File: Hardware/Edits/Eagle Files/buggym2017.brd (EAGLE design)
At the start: 88.9 x 81.3 mm, 6 parts, among them IC1 4001N, IC2 4075N, IC3 BCC, IC4 L293E

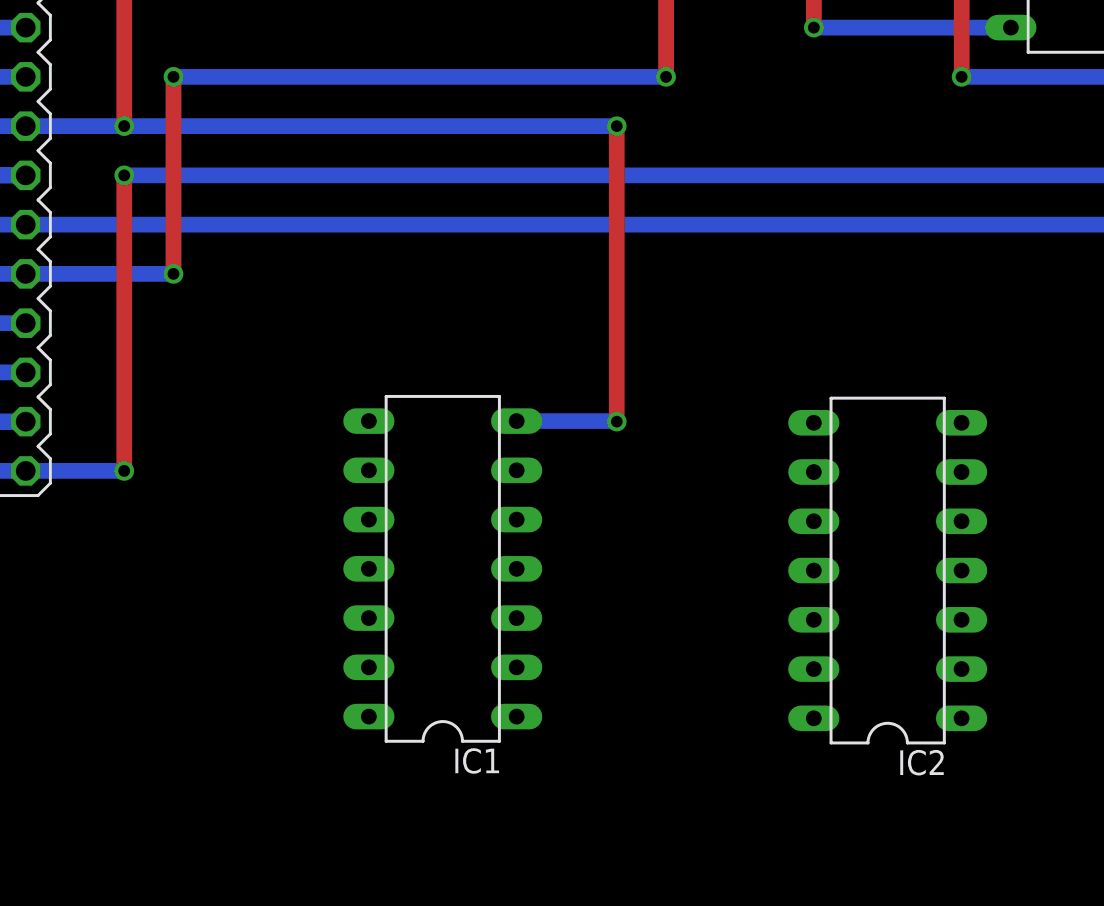
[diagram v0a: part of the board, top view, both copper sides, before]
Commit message: Work Done in Week 3  HardwareLab
Work done in Multisim and Eagle
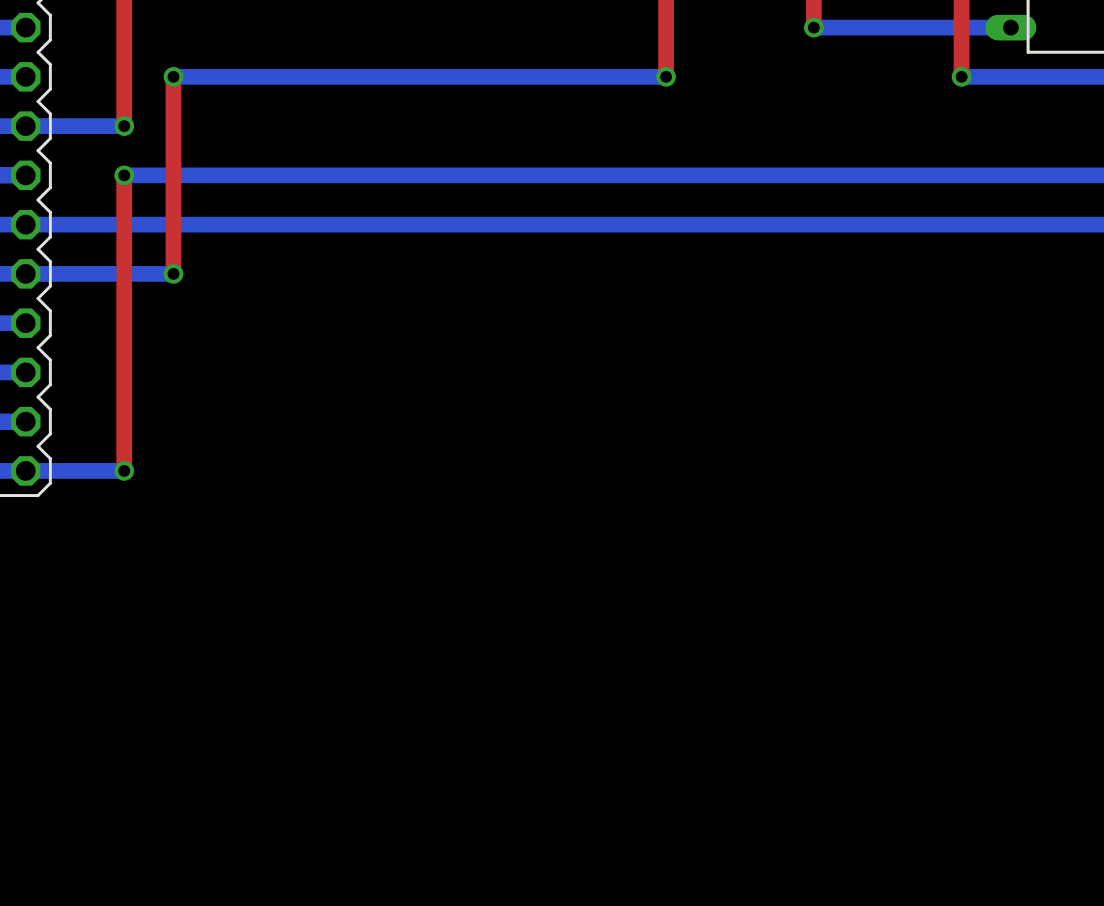
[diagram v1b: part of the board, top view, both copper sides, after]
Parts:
- removed IC1: 4001N, 40xx:DIL14
- removed IC2: 4075N, 40xx:DIL14
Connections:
- removed net LM: IC2.9
- removed net N$1: IC1.3, IC2.2
- removed net N$4: IC1.4, IC2.4
- removed net RM: IC2.6
- removed net VDD: IC1.14, IC2.14
- net GND: no longer IC1.7, IC2.7
- net L_EYE: no longer BUGGY_CON.4
- net R_EYE: no longer BUGGY_CON.3
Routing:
- net GND: track 159.9 -> 94.0 mm, vias 8 -> 6
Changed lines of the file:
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@@
 <?xml version="1.0" encoding="utf-8"?>
 <!DOCTYPE eagle SYSTEM "eagle.dtd">
-<eagle version="7.7.0">
+<eagle version="7.3.0">
 <drawing>
 <settings>
@@
 <setting verticaltext="up"/>
 </settings>
-<grid distance="0.1" unitdist="inch" unit="inch" style="lines" multiple="1" display="yes" altdistance="0.01" altunitdist="inch" altunit="inch"/>
+<grid distance="0.1" unitdist="inch" unit="inch" style="lines" multiple="1" display="yes" altdistance="0.025" altunitdist="inch" altunit="inch"/>
 <layers>
 <layer number="1" name="Top" color="4" fill="1" visible="yes" active="yes"/>
@@
 <layer number="27" name="tValues" color="7" fill="1" visible="yes" active="yes"/>
 <layer number="28" name="bValues" color="7" fill="1" visible="yes" active="yes"/>
-<layer number="29" name="tStop" color="7" fill="3" visible="yes" active="yes"/>
-<layer number="30" name="bStop" color="7" fill="6" visible="yes" active="yes"/>
-<layer number="31" name="tCream" color="7" fill="4" visible="yes" active="yes"/>
-<layer number="32" name="bCream" color="7" fill="5" visible="yes" active="yes"/>
-<layer number="33" name="tFinish" color="6" fill="3" visible="yes" active="yes"/>
-<layer number="34" name="bFinish" color="6" fill="6" visible="yes" active="yes"/>
-<layer number="35" name="tGlue" color="7" fill="4" visible="yes" active="yes"/>
-<layer number="36" name="bGlue" color="7" fill="5" visible="yes" active="yes"/>
-<layer number="37" name="tTest" color="7" fill="1" visible="yes" active="yes"/>
-<layer number="38" name="bTest" color="7" fill="1" visible="yes" active="yes"/>
+<layer number="29" name="tStop" color="7" fill="3" visible="no" active="yes"/>
+<layer number="30" name="bStop" color="7" fill="6" visible="no" active="yes"/>
+<layer number="31" name="tCream" color="7" fill="4" visible="no" active="yes"/>
+<layer number="32" name="bCream" color="7" fill="5" visible="no" active="yes"/>
+<layer number="33" name="tFinish" color="6" fill="3" visible="no" active="yes"/>
+<layer number="34" name="bFinish" color="6" fill="6" visible="no" active="yes"/>
+<layer number="35" name="tGlue" color="7" fill="4" visible="no" active="yes"/>
+<layer number="36" name="bGlue" color="7" fill="5" visible="no" active="yes"/>
+<layer number="37" name="tTest" color="7" fill="1" visible="no" active="yes"/>
+<layer number="38" name="bTest" color="7" fill="1" visible="no" active="yes"/>
 <layer number="39" name="tKeepout" color="4" fill="11" visible="yes" active="yes"/>
 <layer number="40" name="bKeepout" color="1" fill="11" visible="yes" active="yes"/>
@@
 <layer number="42" name="bRestrict" color="1" fill="10" visible="yes" active="yes"/>
 <layer number="43" name="vRestrict" color="2" fill="10" visible="yes" active="yes"/>
-<layer number="44" name="Drills" color="7" fill="1" visible="yes" active="yes"/>
-<layer number="45" name="Holes" color="7" fill="1" visible="yes" active="yes"/>
-<layer number="46" name="Milling" color="3" fill="1" visible="yes" active="yes"/>
-<layer number="47" name="Measures" color="7" fill="1" visible="yes" active="yes"/>
+<layer number="44" name="Drills" color="7" fill="1" visible="no" active="yes"/>
+<layer number="45" name="Holes" color="7" fill="1" visible="no" active="yes"/>
+<layer number="46" name="Milling" color="3" fill="1" visible="no" active="yes"/>
+<layer number="47" name="Measures" color="7" fill="1" visible="no" active="yes"/>
 <layer number="48" name="Document" color="7" fill="1" visible="yes" active="yes"/>
 <layer number="49" name="Reference" color="7" fill="1" visible="yes" active="yes"/>
@@
 </element>
 <element name="BUGGY_CON" library="2E10" package="2E10BOARD" value="2E10HDR" x="26.67" y="38.1"/>
-<element name="IC1" library="40xx" package="DIL14" value="4001N" x="49.44543125" y="17.810665625" rot="R90"/>
-<element name="IC2" library="40xx" package="DIL14" value="4075N" x="72.387890625" y="17.722265625" rot="R90"/>
 </elements>
 <signals>
@@
 <wire x1="27.94" y1="53.34" x2="43.18" y2="53.34" width="0.8128" layer="16"/>
 <via x="45.72" y="53.34" extent="1-16" drill="0.6096" shape="square"/>
-<contactref element="IC1" pad="7"/>
-<contactref element="IC2" pad="7"/>
-<wire x1="33.02" y1="40.64" x2="52.944703125" y2="40.64" width="0.4064" layer="16"/>
-<wire x1="52.944703125" y1="40.64" x2="52.944703125" y2="40.489321875" width="0.4064" layer="16"/>
-<wire x1="53.25543125" y1="25.430665625" x2="58.42" y2="25.430665625" width="0.8128" layer="16"/>
-<wire x1="58.42" y1="25.430665625" x2="58.42" y2="25.4" width="0.8128" layer="16"/>
-<via x="58.42" y="25.4" extent="1-16" drill="0.6" shape="square"/>
-<wire x1="58.42" y1="25.4" x2="58.42" y2="40.64" width="0.8128" layer="1"/>
-<via x="58.42" y="40.64" extent="1-16" drill="0.6" shape="square"/>
-<wire x1="58.42" y1="40.64" x2="33.02" y2="40.64" width="0.8128" layer="16"/>
-<wire x1="58.42" y1="25.430665625" x2="76.197890625" y2="25.342265625" width="0" layer="19" extent="16-16"/>
 </signal>
 <signal name="N$2">
@@
 <signal name="R_EYE">
 <contactref element="BUGGY_CON" pad="3'"/>
-<contactref element="BUGGY_CON" pad="3"/>
 </signal>
 <signal name="L_EYE">
 <contactref element="BUGGY_CON" pad="4'"/>
-<contactref element="BUGGY_CON" pad="4"/>
 </signal>
 <signal name="N$3">
@@
 <wire x1="60.96" y1="53.34" x2="58.42" y2="53.34" width="0.8128" layer="16"/>
 </signal>
-<signal name="VDD">
-<contactref element="IC1" pad="14"/>
-<contactref element="IC2" pad="14"/>
-<wire x1="45.63543125" y1="10.190665625" x2="68.577890625" y2="10.102265625" width="0" layer="19" extent="1-1"/>
-</signal>
-<signal name="N$1">
-<contactref element="IC1" pad="3"/>
-<contactref element="IC2" pad="2"/>
-<wire x1="53.25543125" y1="15.270665625" x2="76.197890625" y2="12.642265625" width="0" layer="19" extent="1-1"/>
-</signal>
-<signal name="LM">
-<contactref element="IC2" pad="9"/>
-</signal>
-<signal name="RM">
-<contactref element="IC2" pad="6"/>
-</signal>
-<signal name="N$4">
-<contactref element="IC1" pad="4"/>
-<contactref element="IC2" pad="4"/>
-<wire x1="53.25543125" y1="17.810665625" x2="76.197890625" y2="17.722265625" width="0" layer="19" extent="1-1"/>
-</signal>
 </signals>
